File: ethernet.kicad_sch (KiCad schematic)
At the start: 51 parts, among them J1 L834-1G1T-S7, U20 KSZ9031RNXCA, Y2 Resonator_25MHz_ABM8G

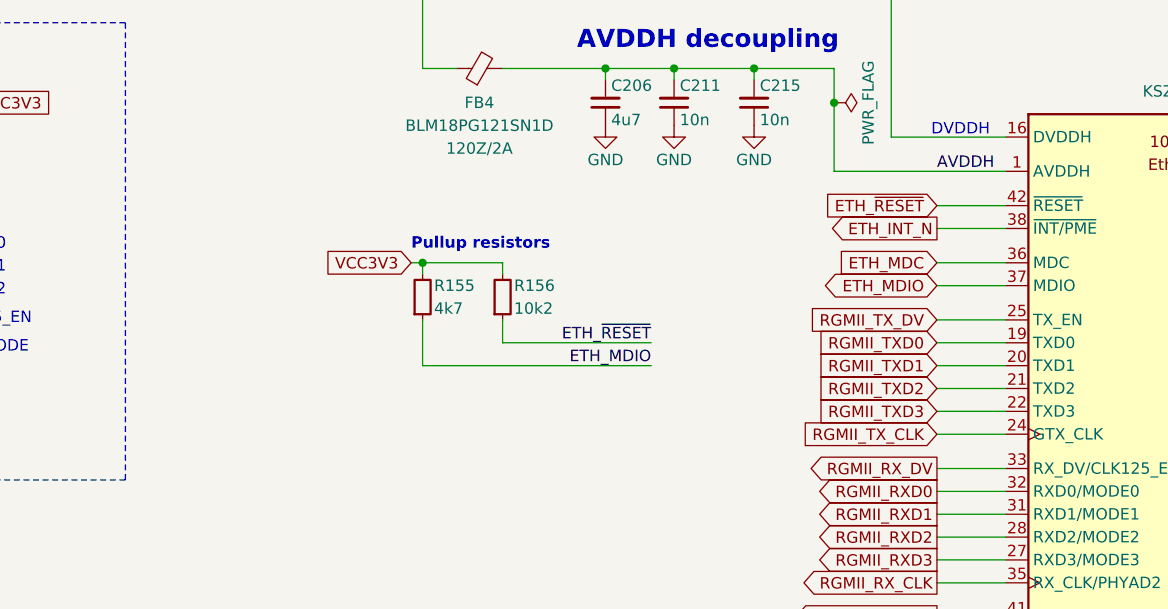
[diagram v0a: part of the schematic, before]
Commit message: pcb layout progress
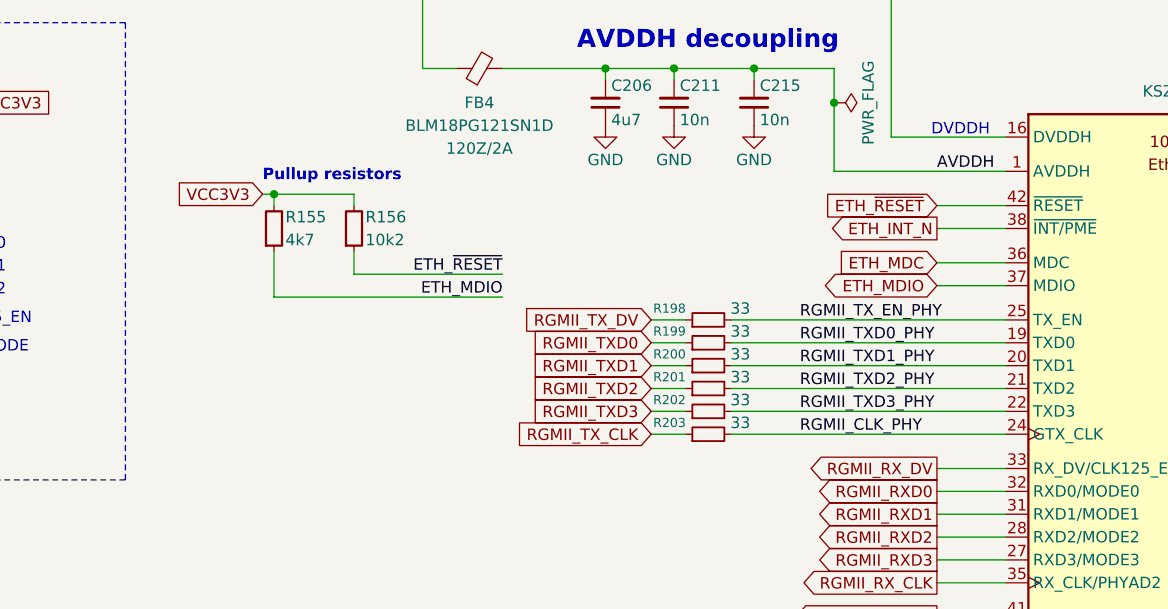
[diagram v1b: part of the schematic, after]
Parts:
- added R198, R199, R200, R201, R202, R203: 33, Resistor_SMD:R_0402_1005Metric, symbol Device:R_Small
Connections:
- net RGMII_TXD0: now also R199.1; no longer U20.19 (TXD0)
- net RGMII_TXD1: now also R200.1; no longer U20.20 (TXD1)
- net RGMII_TXD2: now also R201.1; no longer U20.21 (TXD2)
- net RGMII_TXD3: now also R202.1; no longer U20.22 (TXD3)
- net RGMII_TX_CLK: now also R203.1; no longer U20.24 (GTX_CLK)
- net RGMII_TX_DV: now also R198.1; no longer U20.25 (TX_EN)
- new net RGMII_CLK_PHY: R203.2, U20.24 (GTX_CLK)
- new net RGMII_TXD0_PHY: R199.2, U20.19 (TXD0)
- new net RGMII_TXD1_PHY: R200.2, U20.20 (TXD1)
- new net RGMII_TXD2_PHY: R201.2, U20.21 (TXD2)
- new net RGMII_TXD3_PHY: R202.2, U20.22 (TXD3)
- new net RGMII_TX_EN_PHY: R198.2, U20.25 (TX_EN)
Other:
- moved on the sheet: R155, R156
